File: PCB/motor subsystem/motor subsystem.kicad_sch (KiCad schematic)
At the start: 16 parts, among them U1 MCU_Seeed_XIAO_ESP32-C3

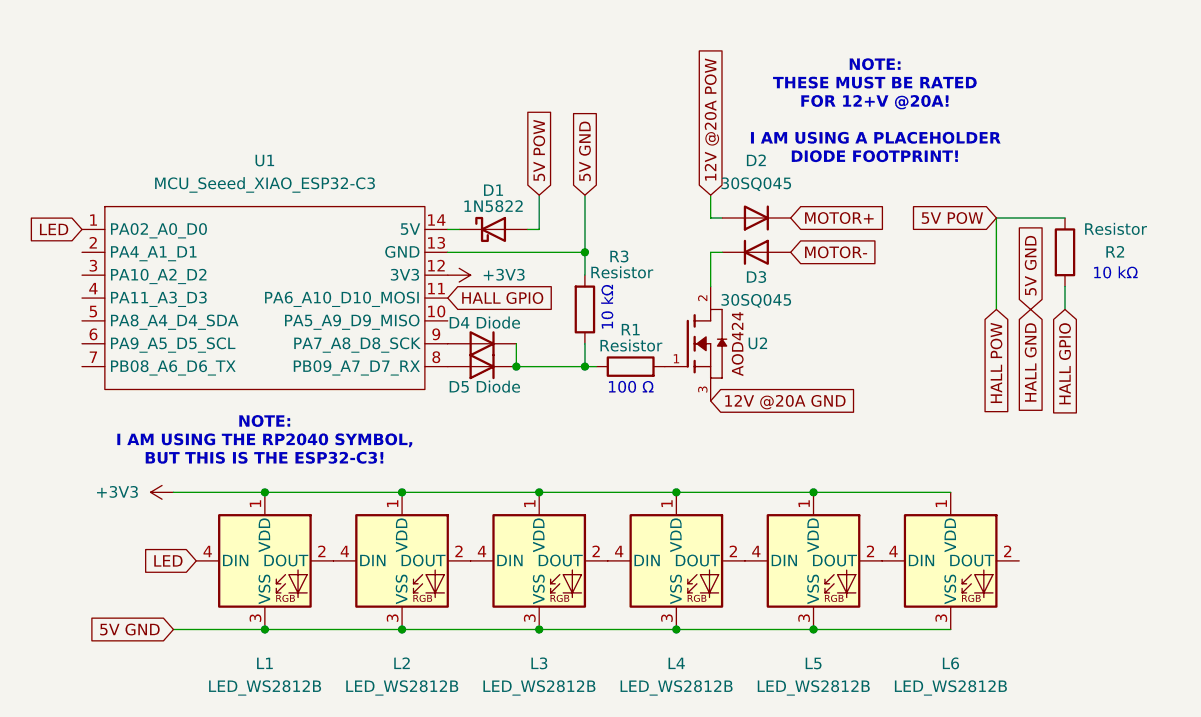
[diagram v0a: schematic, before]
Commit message: motor pcb edits
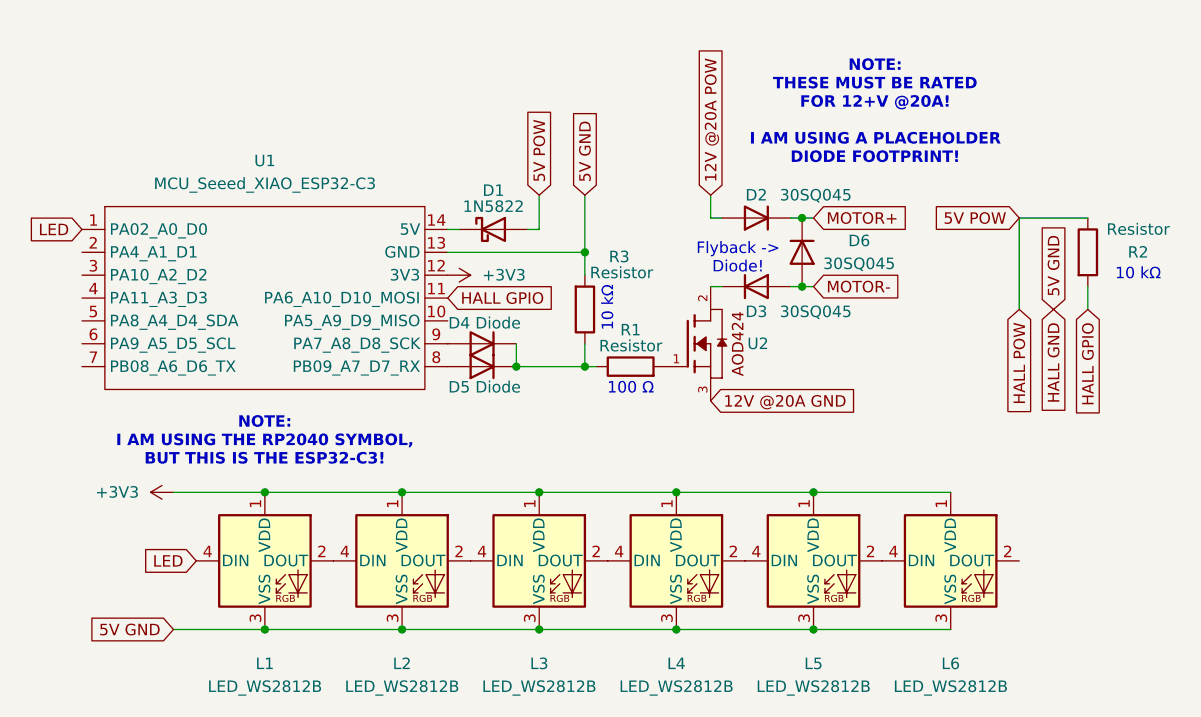
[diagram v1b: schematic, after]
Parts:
- added D6: 30SQ045, Resistor_THT:R_Axial_DIN0918_L18.0mm_D9.0mm_P25.40mm_Horizontal, symbol ScottoKeebs:Placeholder_Diode
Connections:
- net MOTOR+: now also D6.1 (K)
- net MOTOR-: now also D6.2 (A)
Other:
- note added: "Flyback -> Diode!"
- moved on the sheet: D3, R2
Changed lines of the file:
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@@
+	)
+	(junction
+		(at 125.73 50.8)
+		(diameter 0)
+		(color 0 0 0 0)
 	)
 	(junction
@@
 	)
 	(junction
+		(at 125.73 43.18)
+		(diameter 0)
+		(color 0 0 0 0)
+	)
+	(junction
 		(at 127 88.9)
 		(diameter 0)
@@
 	(wire
 		(pts
-			(xy 147.32 43.18) (xy 147.32 53.34)
+			(xy 149.86 43.18) (xy 149.86 53.34)
+		)
+		(stroke
+			(width 0)
+			(type default)
+		)
+	)
+	(wire
+		(pts
+			(xy 125.73 43.18) (xy 124.46 43.18)
 		)
 		(stroke
@@
 	(wire
 		(pts
-			(xy 115.57 46.99) (xy 115.57 50.8)
-		)
-		(stroke
-			(width 0)
-			(type default)
-		)
-	)
-	(wire
-		(pts
 			(xy 96.52 44.45) (xy 95.25 44.45)
 		)
@@
 	(wire
 		(pts
-			(xy 115.57 46.99) (xy 116.84 46.99)
+			(xy 115.57 50.8) (xy 116.84 50.8)
 		)
 		(stroke
@@
 	(wire
 		(pts
-			(xy 154.94 50.8) (xy 154.94 53.34)
+			(xy 157.48 50.8) (xy 157.48 53.34)
 		)
 		(stroke
@@
 	(wire
 		(pts
+			(xy 125.73 43.18) (xy 127 43.18)
+		)
+		(stroke
+			(width 0)
+			(type default)
+		)
+	)
+	(wire
+		(pts
+			(xy 125.73 50.8) (xy 127 50.8)
+		)
+		(stroke
+			(width 0)
+			(type default)
+		)
+	)
+	(wire
+		(pts
 			(xy 111.76 73.66) (xy 127 73.66)
 		)
@@
 	(wire
 		(pts
-			(xy 147.32 43.18) (xy 154.94 43.18)
+			(xy 149.86 43.18) (xy 157.48 43.18)
+		)
+		(stroke
+			(width 0)
+			(type default)
+		)
+	)
+	(wire
+		(pts
+			(xy 124.46 50.8) (xy 125.73 50.8)
 		)
 		(stroke
@@
 	(text "10 kΩ"
 		(exclude_from_sim no)
-		(at 160.528 49.53 0)
+		(at 163.068 49.53 0)
 		(effects
 			(font
@@
 		)
 	)
+	(text "Flyback ->\nDiode!"
+		(exclude_from_sim no)
+		(at 118.618 47.752 0)
+		(effects
+			(font
+				(face "Orbitron")
+				(size 1.27 1.27)
+			)
+		)
+	)
 	(text "100 Ω"
 		(exclude_from_sim no)
@@
 	(global_label "MOTOR-"
 		(shape input)
-		(at 124.46 46.99 0)
+		(at 127 50.8 0)
 		(fields_autoplaced yes)
 		(effects
@@
 		)
 		(property "Intersheetrefs" "${INTERSHEET_REFS}"
-			(at 135.3676 46.99 0)
+			(at 137.9076 50.8 0)
 			(effects
 				(font
@@
 	(global_label "HALL GND"
 		(shape input)
-		(at 151.13 53.34 270)
+		(at 153.67 53.34 270)
 		(fields_autoplaced yes)
 		(effects
@@
 		)
 		(property "Intersheetrefs" "${INTERSHEET_REFS}"
-			(at 151.13 65.6386 90)
+			(at 153.67 65.6386 90)
 			(effects
 				(font
@@
 	(global_label "HALL POW"
 		(shape input)
-		(at 147.32 53.34 270)
+		(at 149.86 53.34 270)
 		(fields_autoplaced yes)
 		(effects
@@
 		)
 		(property "Intersheetrefs" "${INTERSHEET_REFS}"
-			(at 147.32 65.82 90)
+			(at 149.86 65.82 90)
 			(effects
 				(font
@@
 	(global_label "5V POW"
 		(shape input)
-		(at 147.32 43.18 180)
+		(at 149.86 43.18 180)
 		(fields_autoplaced yes)
 		(effects
@@
 		)
 		(property "Intersheetrefs" "${INTERSHEET_REFS}"
-			(at 137.0172 43.18 0)
+			(at 139.5572 43.18 0)
 			(effects
 				(font
@@
 	(global_label "5V GND"
 		(shape input)
-		(at 151.13 53.34 90)
+		(at 153.67 53.34 90)
 		(fields_autoplaced yes)
 		(effects
@@
 		)
 		(property "Intersheetrefs" "${INTERSHEET_REFS}"
-			(at 151.13 43.2186 90)
+			(at 153.67 43.2186 90)
 			(effects
 				(font
@@
 	(global_label "MOTOR+"
 		(shape input)
-		(at 124.46 43.18 0)
+		(at 127 43.18 0)
 		(fields_autoplaced yes)
 		(effects
@@
 		)
 		(property "Intersheetrefs" "${INTERSHEET_REFS}"
-			(at 135.3676 43.18 0)
+			(at 137.9076 43.18 0)
 			(effects
 				(font
@@
 	(global_label "HALL GPIO"
 		(shape input)
-		(at 154.94 53.34 270)
+		(at 157.48 53.34 270)
 		(fields_autoplaced yes)
 		(effects
@@
 		)
 		(property "Intersheetrefs" "${INTERSHEET_REFS}"
-			(at 154.94 66.2434 90)
+			(at 157.48 66.2434 90)
 			(effects
 				(font
@@
 	(symbol
 		(lib_id "ScottoKeebs:Placeholder_Resistor")
-		(at 154.94 46.99 270)
+		(at 157.48 46.99 270)
 		(unit 1)
 		(exclude_from_sim no)
@@
 		(dnp no)
 		(property "Reference" "R2"
-			(at 160.528 46.99 90)
+			(at 163.068 46.99 90)
 			(effects
 				(font
@@
 		)
 		(property "Value" "Resistor"
-			(at 160.528 44.45 90)
+			(at 163.068 44.45 90)
 			(effects
 				(font
@@
 		)
 		(property "Footprint" "Resistor_THT:R_Axial_DIN0411_L9.9mm_D3.6mm_P15.24mm_Horizontal"
-			(at 153.162 46.99 0)
+			(at 155.702 46.99 0)
 			(effects
 				(font
@@
 		)
 		(property "Datasheet" "~"
-			(at 154.94 46.99 90)
+			(at 157.48 46.99 90)
 			(effects
 				(font
@@
 		)
 		(property "Description" "Resistor"
-			(at 154.94 46.99 0)
+			(at 157.48 46.99 0)
 			(effects
 				(font
@@
 	)
 	(symbol
+		(lib_id "ScottoKeebs:Placeholder_Diode")
+		(at 125.73 46.99 270)
+		(unit 1)
+		(exclude_from_sim no)
+		(in_bom yes)
+		(on_board yes)
+		(dnp no)
+		(property "Reference" "D6"
+			(at 132.08 45.72 90)
+			(effects
+				(font
+					(size 1.27 1.27)
+				)
+			)
+		)
+		(property "Value" "30SQ045"
+			(at 132.08 48.26 90)
+			(effects
+				(font
+					(size 1.27 1.27)
+				)
+			)
+		)
+		(property "Footprint" "Resistor_THT:R_Axial_DIN0918_L18.0mm_D9.0mm_P25.40mm_Horizontal"
+			(at 125.73 46.99 0)
+			(effects
+				(font
+					(size 1.27 1.27)
+				)
+				(hide yes)
+			)
+		)
+		(property "Datasheet" ""
+			(at 125.73 46.99 0)
+			(effects
+				(font
+					(size 1.27 1.27)
+				)
+				(hide yes)
+			)
+		)
+		(property "Description" "1N4148 (DO-35) or 1N4148W (SOD-123)"
+			(at 125.73 46.99 0)
+			(effects
+				(font
+					(size 1.27 1.27)
+				)
+				(hide yes)
+			)
+		)
+		(property "Sim.Device" "D"
+			(at 125.73 46.99 0)
+			(effects
+				(font
+					(size 1.27 1.27)
+				)
+				(hide yes)
+			)
+		)
+		(property "Sim.Pins" "1=K 2=A"
+			(at 125.73 46.99 0)
+			(effects
+				(font
+					(size 1.27 1.27)
+				)
+				(hide yes)
+			)
+		)
+		(pin "1"
+		)
+		(pin "2"
+		)
+		(instances
+			(project "motor subsystem"
+				(path "/4cf0086b-fa07-4566-99be-a226804ba080"
+					(reference "D6")
+					(unit 1)
+				)
+			)
+		)
+	)
+	(symbol
 		(lib_id "ScottoKeebs:LED_WS2812B")
 		(at 66.04 81.28 0)
@@
 		(on_board yes)
 		(dnp no)
-		(fields_autoplaced yes)
 		(property "Reference" "D2"
-			(at 120.65 36.83 0)
+			(at 120.65 40.64 0)
 			(effects
 				(font
@@
 		)
 		(property "Value" "30SQ045"
-			(at 120.65 39.37 0)
+			(at 127.254 40.64 0)
 			(effects
 				(font
@@
 	(symbol
 		(lib_id "ScottoKeebs:Placeholder_Diode")
-		(at 120.65 46.99 0)
+		(at 120.65 50.8 0)
 		(unit 1)
 		(exclude_from_sim no)
@@
 		(dnp no)
 		(property "Reference" "D3"
-			(at 120.65 49.784 0)
+			(at 120.65 53.594 0)
 			(effects
 				(font
@@
 		)
 		(property "Value" "30SQ045"
-			(at 120.65 52.324 0)
+			(at 127.254 53.594 0)
 			(effects
 				(font
@@
 		)
 		(property "Footprint" "Resistor_THT:R_Axial_DIN0918_L18.0mm_D9.0mm_P25.40mm_Horizontal"
-			(at 120.65 46.99 0)
+			(at 120.65 50.8 0)
 			(effects
 				(font
@@
 		)
 		(property "Datasheet" ""
-			(at 120.65 46.99 0)
+			(at 120.65 50.8 0)
 			(effects
 				(font
@@
 		)
 		(property "Description" "1N4148 (DO-35) or 1N4148W (SOD-123)"
-			(at 120.65 46.99 0)
+			(at 120.65 50.8 0)
 			(effects
 				(font
@@
 		)
 		(property "Sim.Device" "D"
-			(at 120.65 46.99 0)
+			(at 120.65 50.8 0)
 			(effects
 				(font
@@
 		)
 		(property "Sim.Pins" "1=K 2=A"
-			(at 120.65 46.99 0)
-			(effects
-				(font
+			(at 120.65 50.8 0)
+			(effects
+				(font
